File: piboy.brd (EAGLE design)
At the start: 76.2 x 76.2 mm, 71 parts, among them CN4 MicroUSB, T1 MMUN2133LT1G, U1 TPS61090RSAR, U2 MCP73871

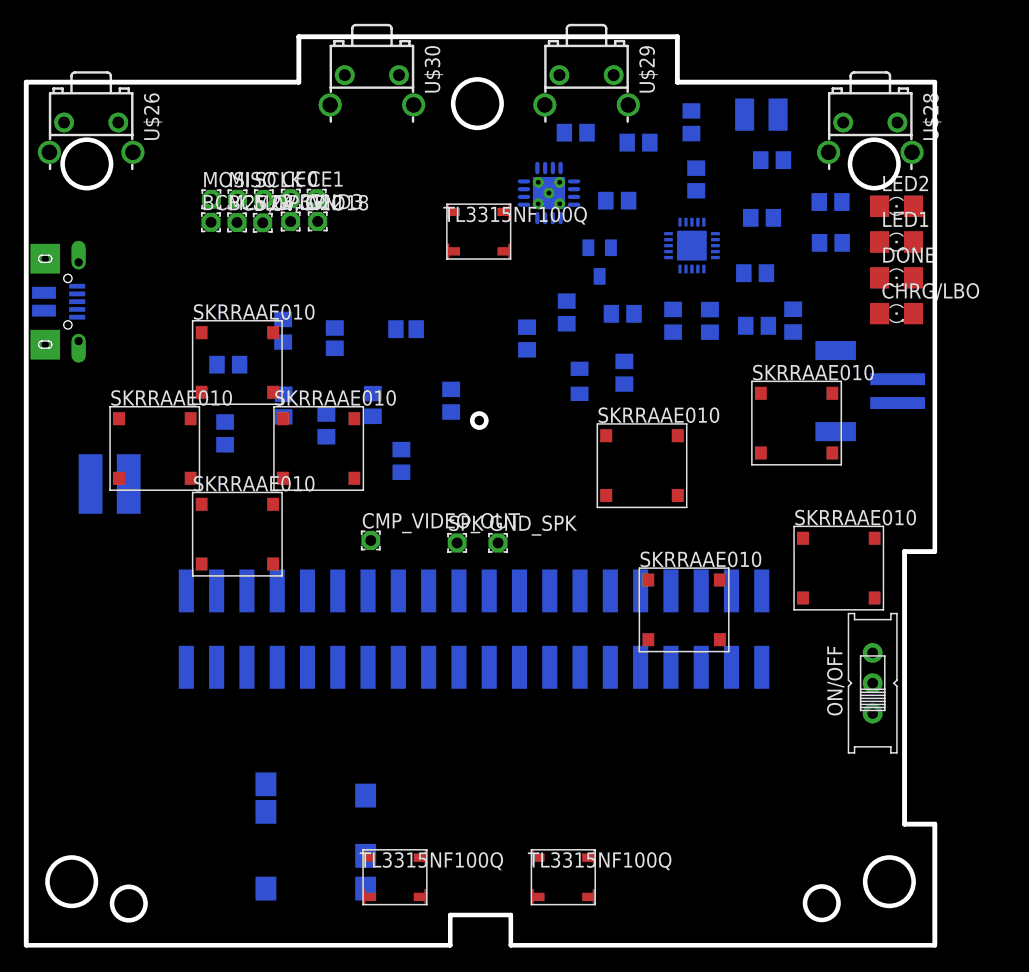
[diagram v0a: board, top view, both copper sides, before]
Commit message: -whoops forgot to save
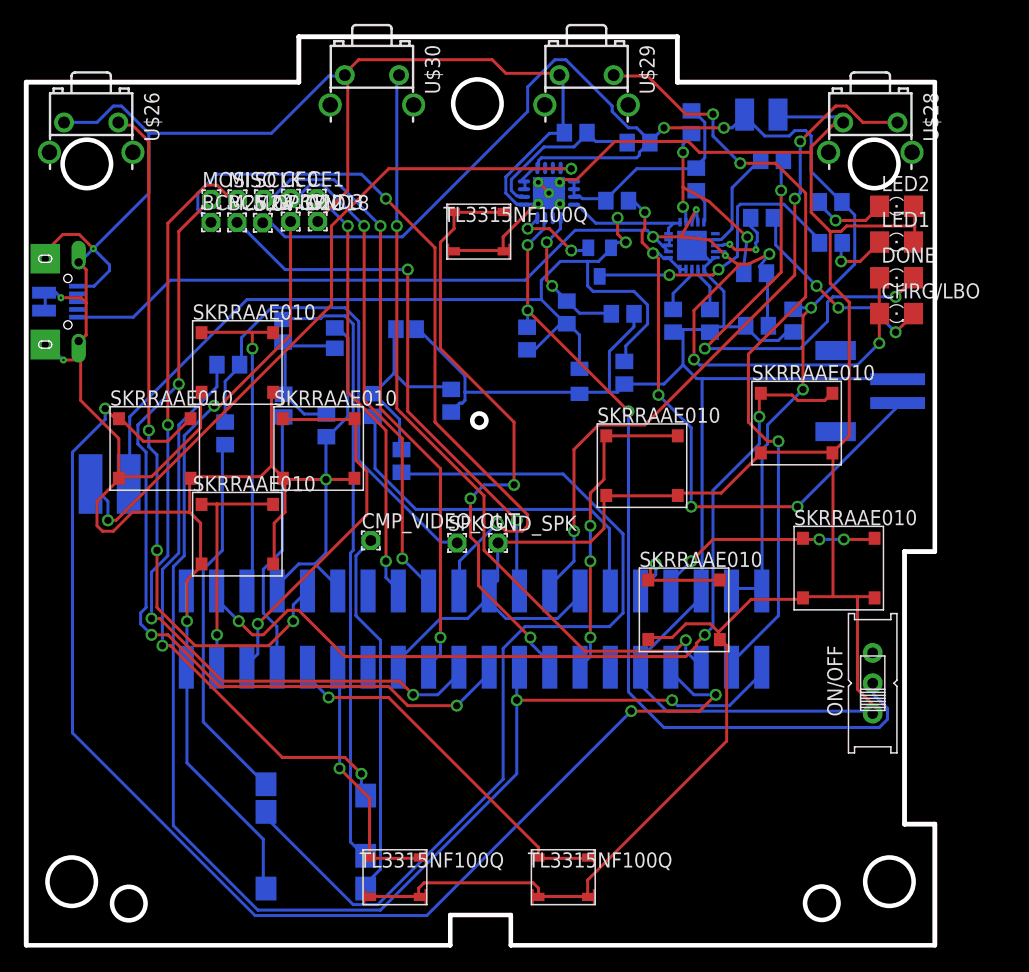
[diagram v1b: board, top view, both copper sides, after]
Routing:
- net GND: track 0.00 -> 635.0 mm, vias 0 -> 5
- net 3.3V: track 0.00 -> 123.1 mm, vias 0 -> 3
- net 5.0V: track 0.00 -> 119.7 mm, vias 0 -> 4
- net J_LFT: track 0.00 -> 110.4 mm, vias 0 -> 3
- net VBUS: track 0.00 -> 109.4 mm, vias 0 -> 6
- net VBAT: track 0.00 -> 92.8 mm, vias 0 -> 2
- net LEFT_HDPHN: track 0.00 -> 77.4 mm
- net J_X: track 0.00 -> 74.9 mm, vias 0 -> 3
- net MOSI: track 0.00 -> 72.5 mm, vias 0 -> 3
- net ENABLE: track 0.00 -> 72.1 mm, vias 0 -> 3
- net MISO: track 0.00 -> 71.1 mm, vias 0 -> 3
- net J_VDN: track 0.00 -> 66.6 mm, vias 0 -> 2
- net J_VUP: track 0.00 -> 66.4 mm, vias 0 -> 3
- net TFT_DC_3V: track 0.00 -> 62.6 mm, vias 0 -> 2
- net N$1: track 0.00 -> 60.2 mm, vias 0 -> 2
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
